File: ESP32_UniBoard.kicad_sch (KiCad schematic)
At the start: 21 parts, among them J1 USB_C_Receptacle_USB2.0, J2 Conn_01x06_Socket, J3 Hirose DF40C, SW1 SW_Push, SW2 SW_Push, U1 ESP32-S3-WROOM-1, U2 SPX3819M5-L-3-3

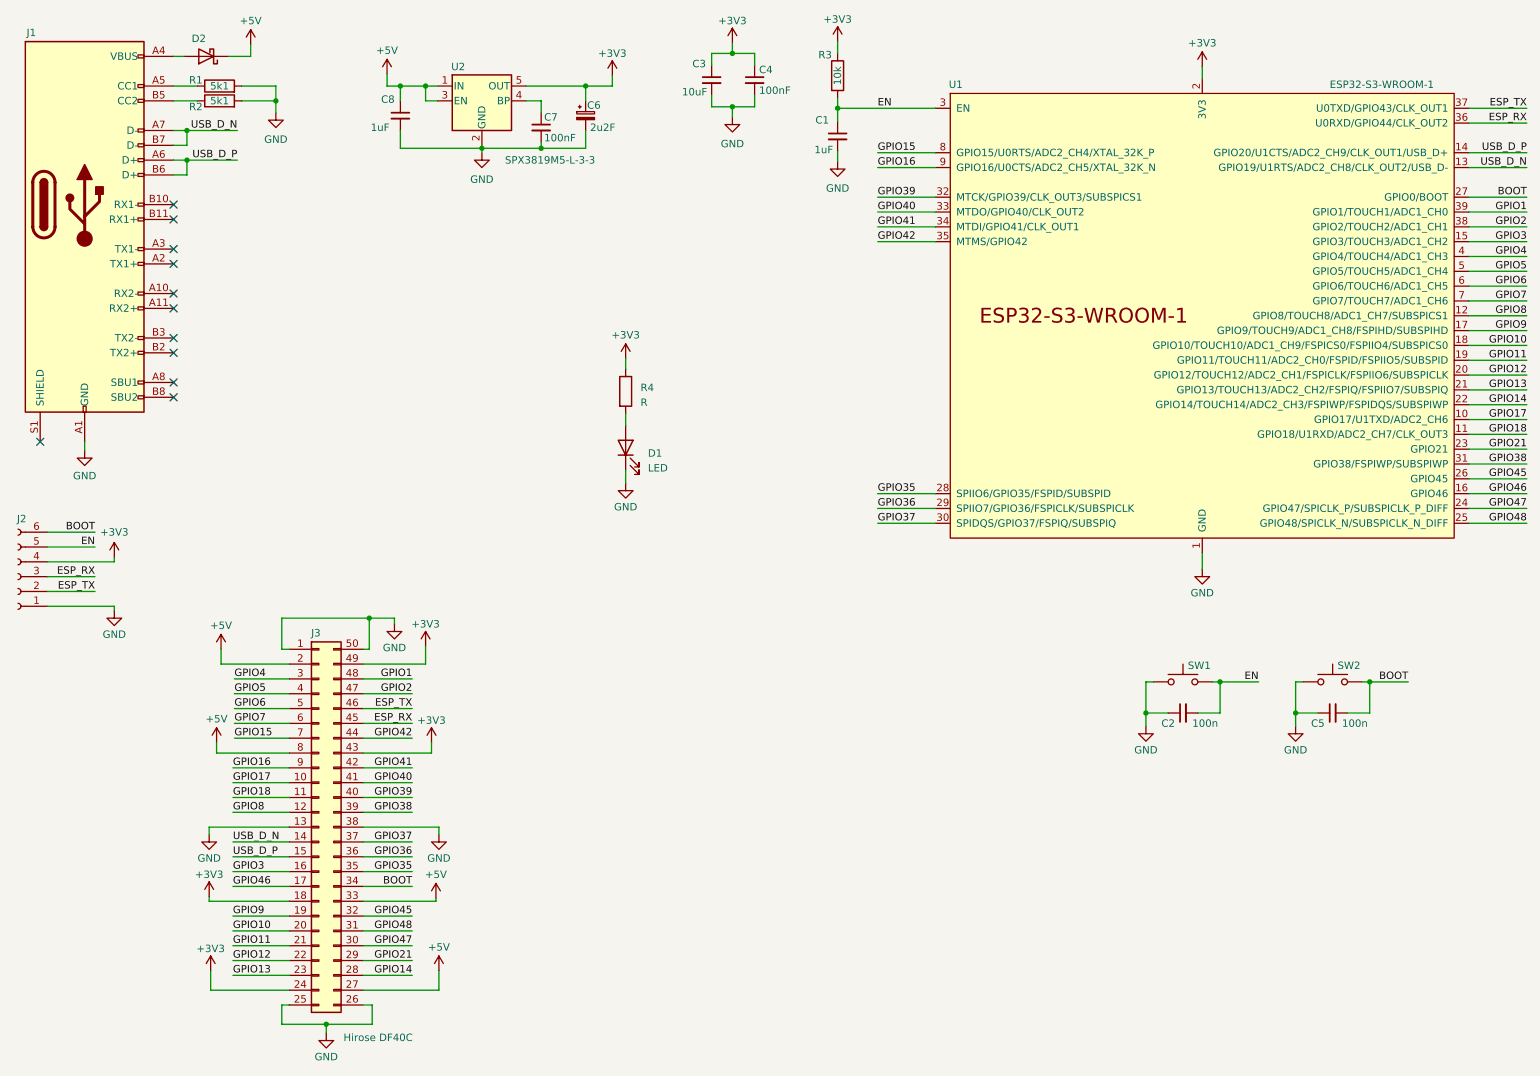
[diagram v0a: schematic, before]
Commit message: Schematics and PCB updates
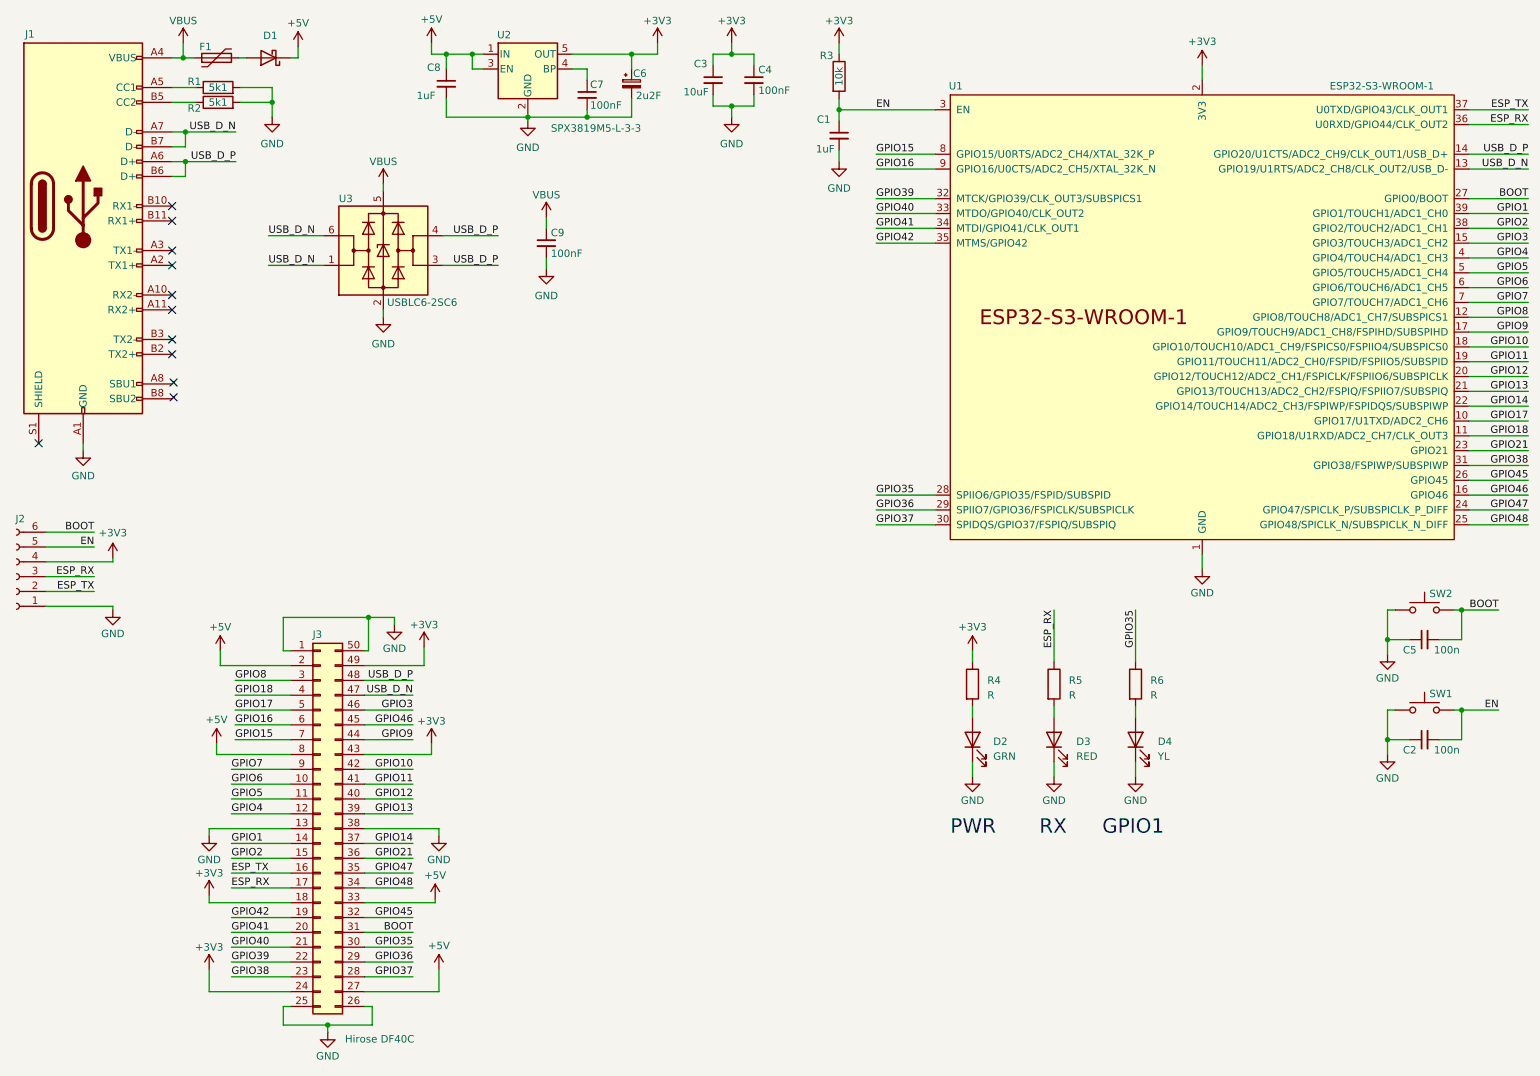
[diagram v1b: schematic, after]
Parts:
- added C9: 100nF, Capacitor_SMD:C_0603_1608Metric_Pad1.08x0.95mm_HandSolder, symbol Device:C_Small
- added D3: RED, LED_SMD:LED_0603_1608Metric_Pad1.05x0.95mm_HandSolder, symbol Device:LED
- added D4: YL, LED_SMD:LED_0603_1608Metric_Pad1.05x0.95mm_HandSolder, symbol Device:LED
- added F1: Polyfuse, Fuse:Fuse_1206_3216Metric_Pad1.42x1.75mm_HandSolder, symbol Device:Polyfuse
- added R5, R6: R, Resistor_SMD:R_0603_1608Metric_Pad0.98x0.95mm_HandSolder, symbol Device:R
- added U3: USBLC6-2SC6, Package_TO_SOT_SMD:SOT-23-6, symbol Power_Protection:USBLC6-2SC6
- D2: renamed from D1; value LED -> GRN
- renumbered D2 to D1
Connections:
- net BOOT: now also J3.31 (Pin_31); no longer J3.34 (Pin_34)
- net ESP_RX: now also J3.17 (Pin_17), R5.1; no longer J3.45 (Pin_45)
- net ESP_TX: now also J3.16 (Pin_16); no longer J3.46 (Pin_46)
- net GND: now also C9.2, D3.1 (K), D4.1 (K), U3.2 (GND)
- net GPIO1: now also J3.14 (Pin_14); no longer J3.48 (Pin_48)
- net GPIO10: now also J3.42 (Pin_42); no longer J3.20 (Pin_20)
- net GPIO11: now also J3.41 (Pin_41); no longer J3.21 (Pin_21)
- net GPIO12: now also J3.40 (Pin_40); no longer J3.22 (Pin_22)
- net GPIO13: now also J3.39 (Pin_39); no longer J3.23 (Pin_23)
- net GPIO14: now also J3.37 (Pin_37); no longer J3.28 (Pin_28)
- net GPIO16: now also J3.6 (Pin_6); no longer J3.9 (Pin_9)
- net GPIO17: now also J3.5 (Pin_5); no longer J3.10 (Pin_10)
- net GPIO18: now also J3.4 (Pin_4); no longer J3.11 (Pin_11)
- net GPIO2: now also J3.15 (Pin_15); no longer J3.47 (Pin_47)
- net GPIO21: now also J3.36 (Pin_36); no longer J3.29 (Pin_29)
- net GPIO3: now also J3.46 (Pin_46); no longer J3.16 (Pin_16)
- net GPIO35: now also J3.30 (Pin_30), R6.1; no longer J3.35 (Pin_35)
- net GPIO36: now also J3.29 (Pin_29); no longer J3.36 (Pin_36)
- net GPIO37: now also J3.28 (Pin_28); no longer J3.37 (Pin_37)
- net GPIO38: now also J3.23 (Pin_23); no longer J3.39 (Pin_39)
- net GPIO39: now also J3.22 (Pin_22); no longer J3.40 (Pin_40)
- net GPIO4: now also J3.12 (Pin_12); no longer J3.3 (Pin_3)
- net GPIO40: now also J3.21 (Pin_21); no longer J3.41 (Pin_41)
- net GPIO41: now also J3.20 (Pin_20); no longer J3.42 (Pin_42)
- net GPIO42: now also J3.19 (Pin_19); no longer J3.44 (Pin_44)
- net GPIO46: now also J3.45 (Pin_45); no longer J3.17 (Pin_17)
- net GPIO47: now also J3.35 (Pin_35); no longer J3.30 (Pin_30)
- net GPIO48: now also J3.34 (Pin_34); no longer J3.31 (Pin_31)
- net GPIO5: now also J3.11 (Pin_11); no longer J3.4 (Pin_4)
- net GPIO6: now also J3.10 (Pin_10); no longer J3.5 (Pin_5)
- net GPIO7: now also J3.9 (Pin_9); no longer J3.6 (Pin_6)
- net GPIO8: now also J3.3 (Pin_3); no longer J3.12 (Pin_12)
- net GPIO9: now also J3.44 (Pin_44); no longer J3.19 (Pin_19)
- net USB_D_N: now also J3.47 (Pin_47), U3.1 (I/O1), U3.6 (I/O1); no longer J3.14 (Pin_14)
- net USB_D_P: now also J3.48 (Pin_48), U3.3 (I/O2), U3.4 (I/O2); no longer J3.15 (Pin_15)
- net VBUS: now reaches J1.A4 (VBUS), J1.A9 (VBUS), J1.B4 (VBUS), J1.B9 (VBUS)
- net VBUS: now also C9.1, F1.1, U3.5 (VBUS); no longer D1.2 (A)
- new net: D1.2 (A), F1.2
- new net: D3.2 (A), R5.2
- new net: D4.2 (A), R6.2
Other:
- note added: "GPIO1"
- note added: "PWR"
- note added: "RX"
- moved on the sheet: C2, C5, C6, C7, C8, D1, D2, R4, SW1, SW2, U2
